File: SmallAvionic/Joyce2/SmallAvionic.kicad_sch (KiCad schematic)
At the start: 103 parts, among them J1 Conn_01x02, J2 Boot_mode_pin, J3 Conn_01x04, J4 USB_C_Receptacle_USB2.0_16P, J5 Conn_01x03, J6 Conn_01x04, J7 Screw_Terminal_01x01, J8 Conn_01x03, Q1 TSM3481CX6 RFG, Q2 TSM3481CX6 RFG, Q3 NMOS, SW1 SW_Push, SW2 USER_Buttom, U1 LD1117S33TR_SOT223, U2 STM32F103C8Tx, U3 LTC4412xS6, U4 TPS54538RQFR, U5 MMC5983MA, U6 BMP390, U7 W25Q128JVS, U8 BMI088, Y1 8Mhz

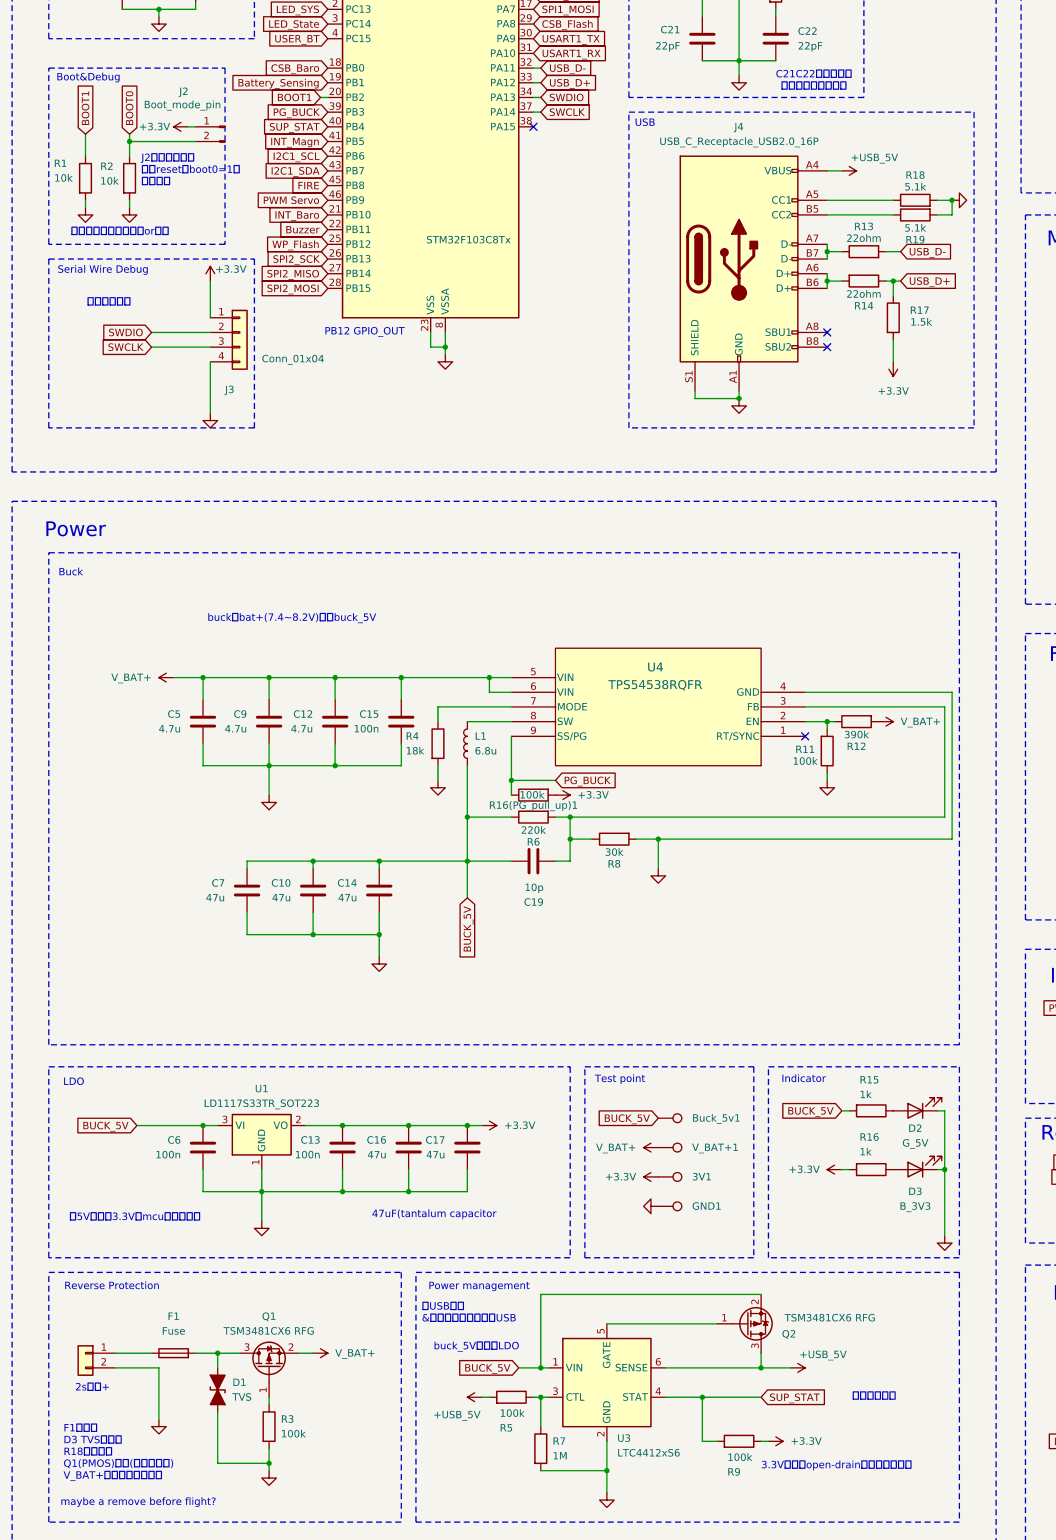
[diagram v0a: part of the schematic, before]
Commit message: new small avionic
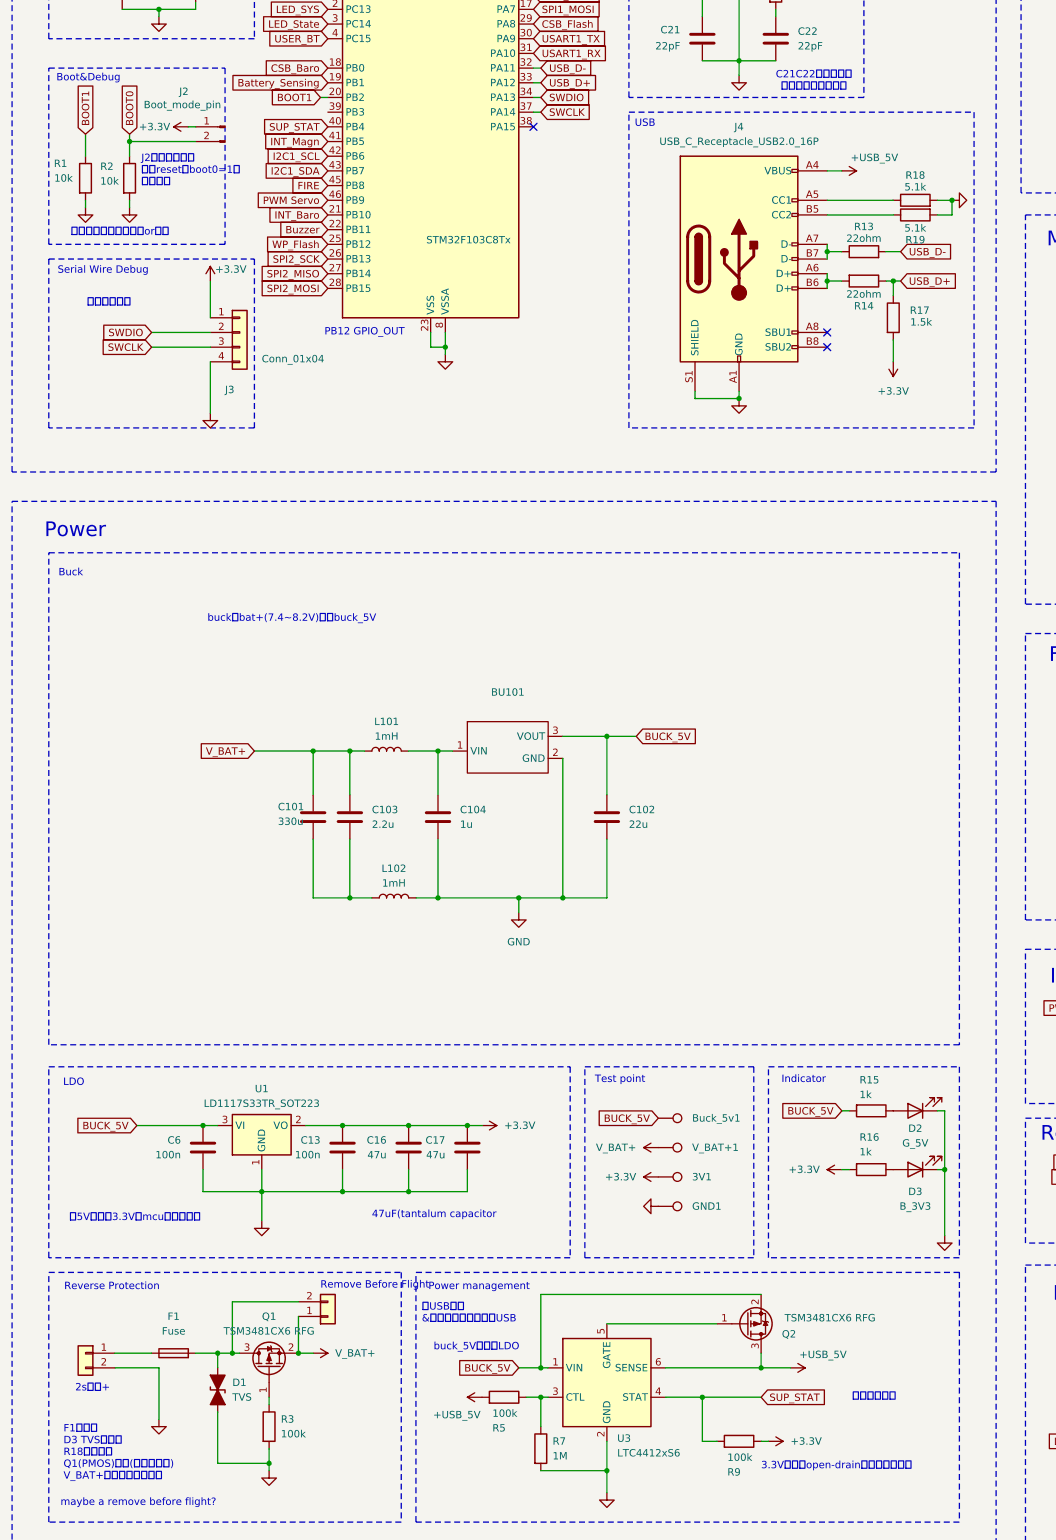
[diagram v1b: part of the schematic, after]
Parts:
- removed C10, C14, C7: 47u, Capacitor_SMD:C_0805_2012Metric_Pad1.18x1.45mm_HandSolder, symbol Device:C
- removed C12, C5, C9: 4.7u, Capacitor_SMD:C_0805_2012Metric_Pad1.18x1.45mm_HandSolder, symbol Device:C
- removed C15: 100n, Capacitor_SMD:C_0805_2012Metric_Pad1.18x1.45mm_HandSolder, symbol Device:C
- removed C19: 10p, Capacitor_SMD:C_0805_2012Metric_Pad1.18x1.45mm_HandSolder, symbol Device:C
- removed L1: 6.8u, Inductor_SMD:L_0805_2012Metric_Pad1.05x1.20mm_HandSolder, symbol Device:L
- removed R11, R16(PG_pull_up)1: 100k, Resistor_SMD:R_0805_2012Metric_Pad1.20x1.40mm_HandSolder, symbol Device:R
- removed R12: 390k, Resistor_SMD:R_0805_2012Metric_Pad1.20x1.40mm_HandSolder, symbol Device:R
- removed R4: 18k, Resistor_SMD:R_0805_2012Metric_Pad1.20x1.40mm_HandSolder, symbol Device:R
- removed R6: 220k, Resistor_SMD:R_0805_2012Metric_Pad1.20x1.40mm_HandSolder, symbol Device:R
- removed R8: 30k, Resistor_SMD:R_0805_2012Metric_Pad1.20x1.40mm_HandSolder, symbol Device:R
- removed U4: TPS54538RQFR, Small_av_joyce_lib:VQFN-HR9_RQF_TEX, symbol Small_av_tony_lib:TPS54538RQFR
- added BU101: ~, Connector:FanPinHeader_1x03_P2.54mm_Vertical, symbol New_Library_0:BK
- added C101: 330u, Capacitor_SMD:C_0805_2012Metric_Pad1.18x1.45mm_HandSolder, symbol Device:C
- added C102: 22u, Capacitor_SMD:C_0805_2012Metric_Pad1.18x1.45mm_HandSolder, symbol Device:C
- added C103: 2.2u, Capacitor_SMD:C_0805_2012Metric_Pad1.18x1.45mm_HandSolder, symbol Device:C
- added C104: 1u, Capacitor_SMD:C_0805_2012Metric_Pad1.18x1.45mm_HandSolder, symbol Device:C
- added J9: Conn_01x02, Connector_JST:JST_EH_B2B-EH-A_1x02_P2.50mm_Vertical, symbol Connector_Generic:Conn_01x02
- added L101, L102: 1mH, Inductor_SMD:L_0805_2012Metric_Pad1.05x1.20mm_HandSolder, symbol Device:L
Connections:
- net BUCK_5V: now also BU101.3 (VOUT), C102.1
- net GND: now also BU101.2 (GND), C102.2, C104.2, L102.2
- net V_BAT+: now also C101.1, C103.1, J9.1 (Pin_1), L101.1
- net at D1.2 (A2), F1.2, Q1.3 (D): now also J9.2 (Pin_2)
- net PG_BUCK: no longer names the net of U2.39 (PB3)
- new net: BU101.1 (VIN), C104.1, L101.2
- new net: C101.2, C103.2, L102.1
- no-connect marks 6 -> 5
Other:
- note added: "Remove Before Flight"
- moved on the sheet: R5
